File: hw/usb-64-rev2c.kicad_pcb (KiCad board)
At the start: 4 copper layers, 69.2 x 46.5 mm, 64 parts, among them J1 USB_C_Receptacle_PowerOnly_6P, J100 Conn_01x03_Pin, J2 USB_C_Receptacle_USB2.0_14P, J3 USB_C_Receptacle_USB2.0_14P, J300 DE9_Receptacle, J301 DE9_Receptacle, SW1 SW_Push, SW2 SW_Push, U100 NCP1117-3.3, U200 RP2040, U201 W25Q128JVSIQ, U300 74AHCT1G125, U301 74AHCT1G125, U302 74AHCT1G125, U303 74AHCT1G125, U304 74AHCT1G125, U305 74AHCT1G125, U306 74AHCT1G125, U307 74AHCT1G125, U308 74AHCT1G125, U309 74AHCT1G125, X100 ASE-12MHz

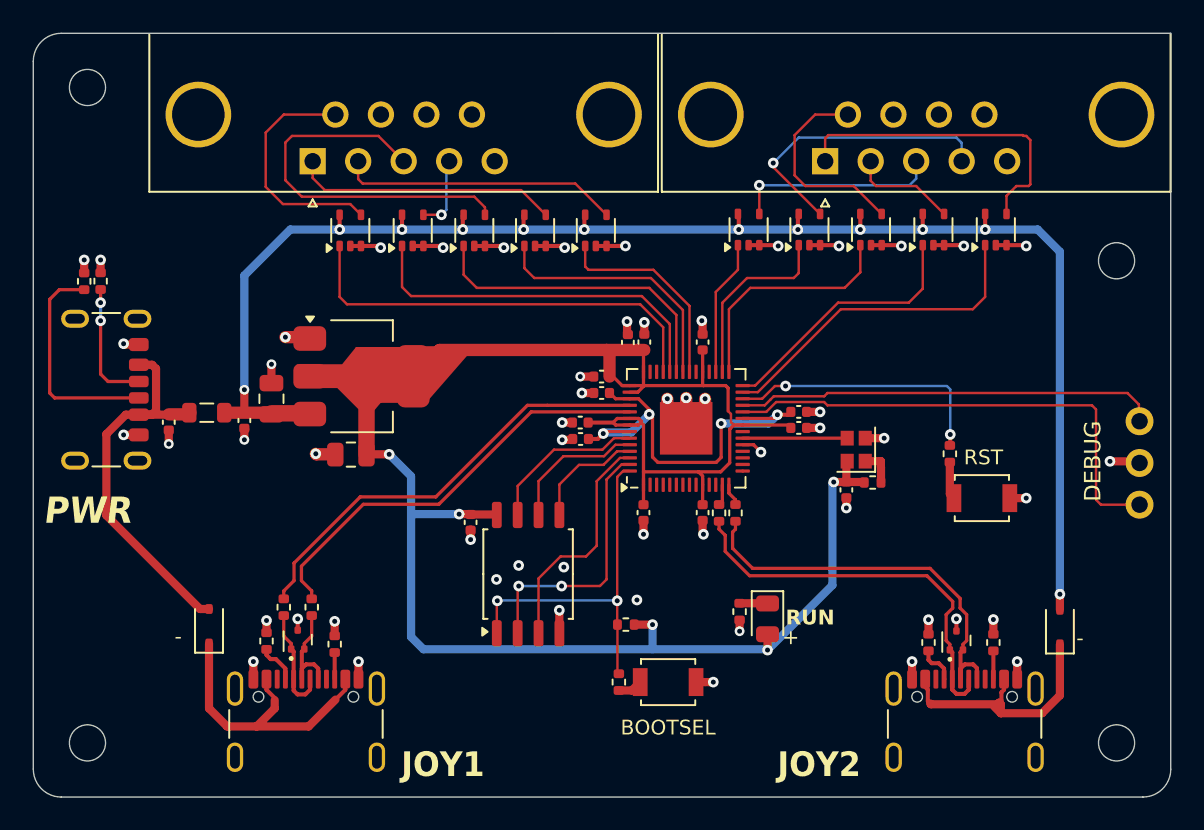
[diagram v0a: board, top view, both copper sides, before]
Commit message: rerouted
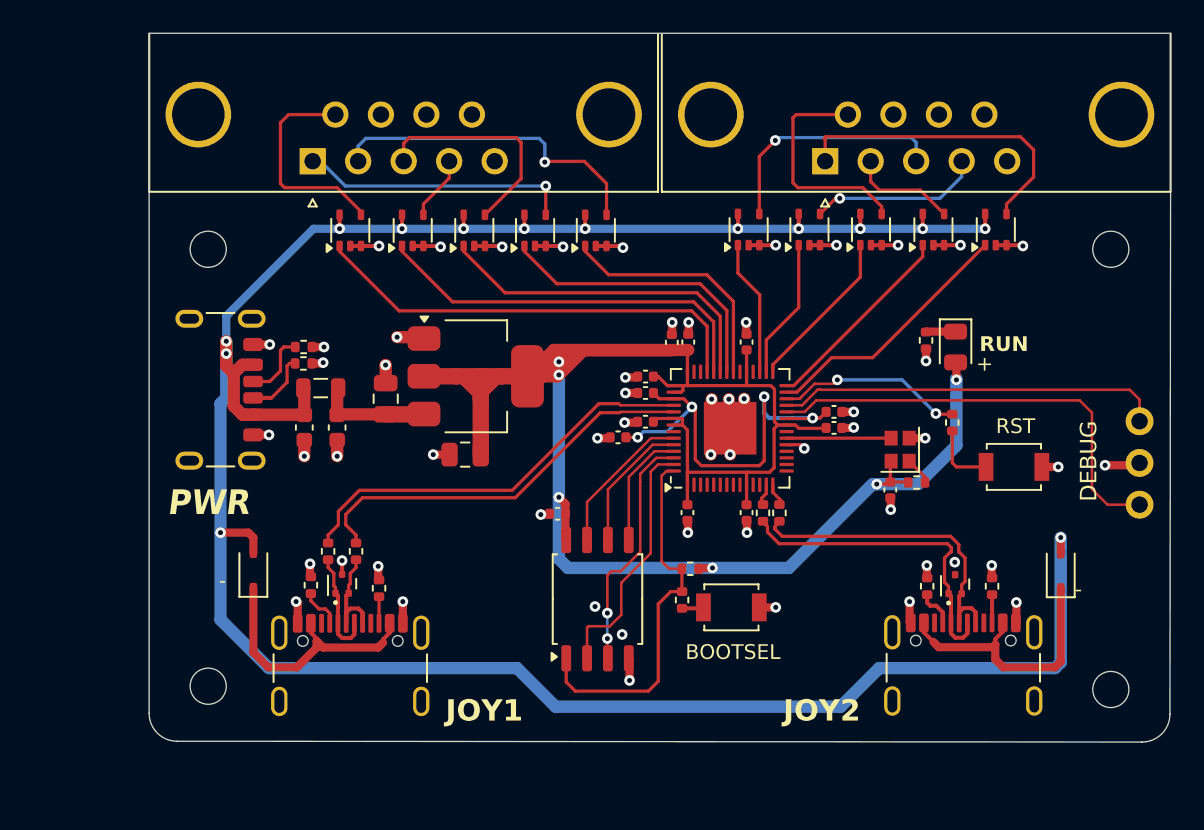
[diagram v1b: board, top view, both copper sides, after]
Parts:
- C5, C6: footprint Capacitor_SMD:C_0402_1005Metric -> Capacitor_SMD:C_0603_1608Metric
- moved H4 62.9 mm to (119.7, 62.1)
- moved H3 62.4 mm to (174.6, 89.0)
- moved H1 37.2 mm to (119.7, 88.8)
- moved D1 20.1 mm to (165.2, 68.1)
- moved R1 20.0 mm to (163.3, 67.7)
- moved R7 14.3 mm to (125.5, 69.1), turned to 0 degrees
- moved R8 13.0 mm to (125.5, 68.1), turned to 0 degrees
- moved C5 8.26 mm to (125.5, 73.0)
- moved FB3 7.10 mm to (126.5, 70.6)
- moved C100 6.96 mm to (130.5, 71.2)
- moved U100 6.96 mm to (135.9, 69.9)
- moved J1 6.95 mm to (119.3, 70.7)
- moved C101 6.95 mm to (135.3, 74.7)
- moved R203 6.31 mm to (148.5, 83.5)
- moved SW1 5.96 mm to (151.5, 84.0)
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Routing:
- net VBUS: track 120.3 -> 161.6 mm, vias 12 -> 14
- net /C64_controls/JOY1_LEFT: track 23.6 -> 13.8 mm
- net Net-(J1-CC2): track 13.6 -> 4.02 mm
- net /C64_controls/JOY2_RIGHT: track 17.6 -> 10.5 mm
- net /MCU/RUN: track 16.5 -> 11.4 mm
- net USB_DEV_D_N: track 26.1 -> 21.2 mm
- net USB_DEV_D_P: track 25.9 -> 21.2 mm
- net IO2_UP: track 20.3 -> 15.8 mm
- net IO2_FIRE: track 14.4 -> 9.92 mm
- net GND: track 60.7 -> 64.7 mm
- net IO2_DOWN: track 16.1 -> 12.2 mm
- net Net-(J1-CC1): track 7.66 -> 4.17 mm, vias 2 -> 0
- net /MCU/SWCLK: track 30.2 -> 27.1 mm
- net IO2_RIGHT: track 11.3 -> 8.53 mm
- net +3.3V: track 124.4 -> 127.1 mm, vias 5 -> 6
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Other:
- board size 69.2 x 46.5 mm -> 62.2 x 43.2 mm
